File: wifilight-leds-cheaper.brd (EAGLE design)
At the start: 50.8 x 50.8 mm, 60 parts, among them Q3 FDN335N, Q4 FDN335N, Q5 FDN335N, Q6 FDN335N, U2 PCA9685

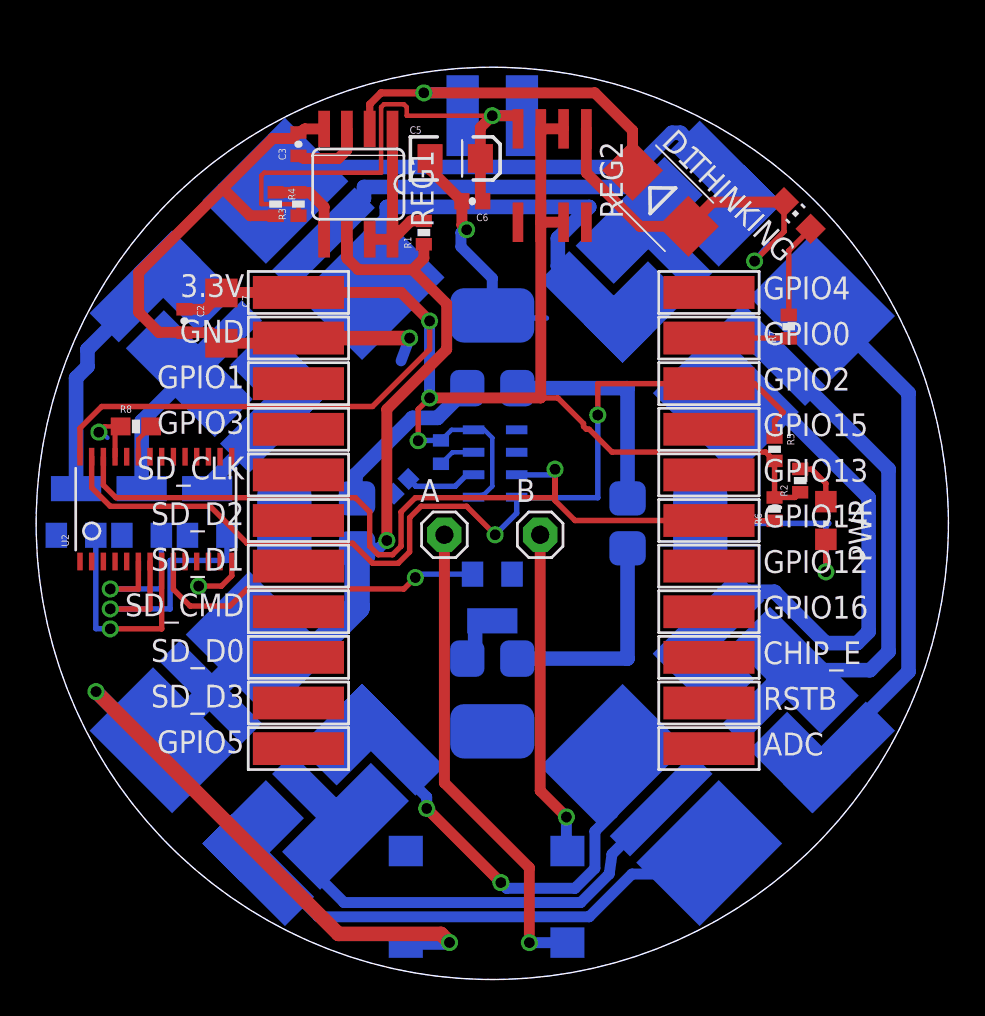
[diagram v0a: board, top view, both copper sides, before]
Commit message: Mk2
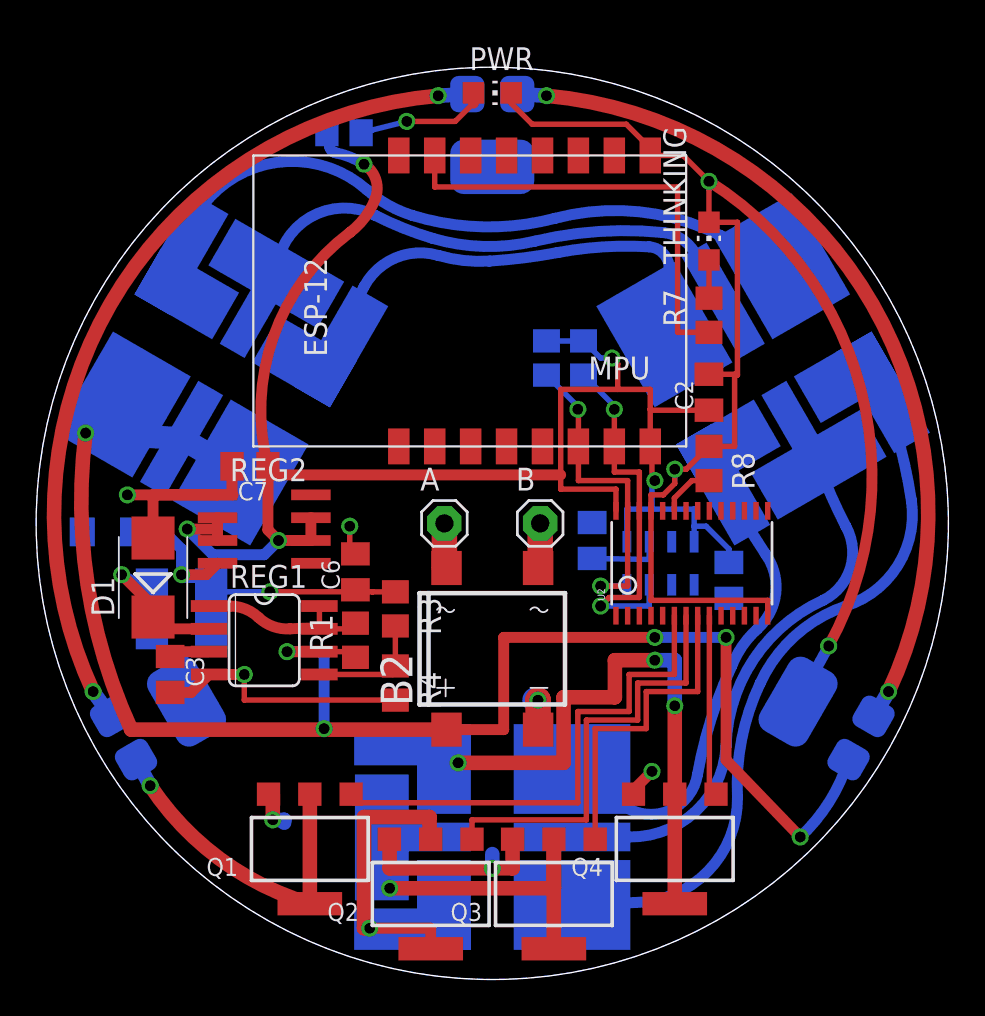
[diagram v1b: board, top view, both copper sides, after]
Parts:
- removed 3.3V, ADC, CHIP_E, GND, GPIO0, GPIO1, GPIO12, GPIO13, GPIO14, GPIO15, GPIO16, GPIO2, GPIO3, GPIO4, GPIO5, RSTB, SD_CLK, SD_CMD, SD_D0, SD_D1, SD_D2, SD_D3: WIREPADSMD5-1,8, wirepad:5-1,8
- removed LED4: OVSTRGBBCR8, led:OVSTRGBBCR8
- removed Q5, Q6: FDN335N, adafruit:SOT23-W
- removed U$4: LUXEON-REBEL, SparkFun-LED:LUXEON-REBEL
- added MPU: ESP8266_ESP-12, ESP8266-ESP12:ESP8266-ESP12
- added Q1, Q2: BUK98180-100A, nxp_60:SOT223
- C1, C2, C3: device SparkFun-Passives:0402-CAP -> resistor:C0805K
- C4, C6: device SparkFun-Capacitors:0402-CAP -> resistor:C0805K
- C7: device SparkFun-Capacitors:1206 -> resistor:C0805K
- Q3, Q4: value FDN335N -> BUK98180-100A; device adafruit:SOT23-W -> nxp_60:SOT223
- R1, R2, R3, R4, R5, R6, R7: device SparkFun-Passives:0402-RES -> resistor:R0805
- R8: device SparkFun-Resistors:0603-RES -> resistor:R0805
- moved D1 35.3 mm to (6.51, 22.4), turned to 90 degrees
- moved LED3 32.5 mm to (25.4, 7.94), turned to 0 degrees
- moved L1 32.5 mm to (8.10, 20.6)
- moved R8 32.0 mm to (37.5, 28.7), turned to 270 degrees
- moved R2 31.9 mm to (17.1, 47.1), flipped to the bottom, turned to 180 degrees
- moved Q3 31.3 mm to (28.8, 4.76), flipped to the top, turned to 180 degrees
- moved C3 30.4 mm to (7.46, 17.0), turned to 270 degrees
- moved U$3 30.3 mm to (7.14, 14.8), turned to 240 degrees
- moved U$1 30.3 mm to (43.7, 14.8), turned to 120 degrees
- moved PWR 30.2 mm to (25.4, 49.4), turned to 270 degrees
- moved U2 30.0 mm to (36.5, 23.2)
- moved C2 29.5 mm to (37.5, 32.7), turned to 90 degrees
- moved C5 28.4 mm to (3.97, 24.9), flipped to the bottom, turned to 180 degrees
- moved R4 27.5 mm to (20.0, 16.5)
- moved REG1 25.9 mm to (12.7, 18.9), turned to 270 degrees
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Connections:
- removed net N$12: U$3.CATHODE, U$4.ANODE
- removed net N$3: LED3.4, LED3.4@1, LED4.1
- removed net N$4: LED3.5, LED3.5@1, LED4.2
- removed net N$9: LED3.6, LED3.6@1, LED4.3
- new net N$25: MPU.13
- new net N$26: MPU.12
- new net N$27: MPU.11
- new net N$28: MPU.10
- new net N$29: MPU.9
- new net N$32: MPU.6
- new net N$33: MPU.4
- new net N$34: MPU.3
- new net N$35: MPU.2
- new net N$36: MPU.5
- net 3.3V: now also MPU.16; no longer 3.3V.1
- net BLUE: now also Q2.1; no longer Q5.1
- net GND: now also MPU.1, Q1.3, Q2.3, Q3.3, Q4.3; no longer GND.1, Q3.2, Q4.2, Q5.2, Q6.2, U$4.P$3
- net GREEN: now also Q4.1, U2.9; no longer Q6.1, U2.8
- net P_BLUE: now also LED3.6, LED3.6@1, Q2.2, Q2.4; no longer LED4.6, LED4.6@1, Q5.3
- net P_GREEN: now also LED3.4, LED3.4@1, Q4.2, Q4.4; no longer LED4.4, LED4.4@1, Q6.3
- net P_RED: now also LED3.5, LED3.5@1, Q3.2, Q3.4; no longer LED4.5, LED4.5@1, Q3.3
- net P_WHITE: now also Q1.2, Q1.4, U$3.CATHODE; no longer Q4.3, U$4.CATHODE
- net RED: now also U2.8; no longer U2.6
- net RESET: now also MPU.8; no longer GPIO4.1
- net SCL: now also MPU.15; no longer GPIO14.1
- net SDA: now also MPU.14; no longer GPIO2.1
- net THINKING: now also MPU.7; no longer GPIO0.1
- net WHITE: now also Q1.1, U2.6; no longer Q4.1, U2.9
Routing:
- net SDA: track 55.1 -> 18.3 mm
- net GND: track 92.9 -> 129.0 mm, vias 6 -> 10
- net 12V: track 77.6 -> 110.6 mm, vias 3 -> 6
- net N$10: track 9.60 -> 41.5 mm, vias 0 -> 2
- net SCL: track 50.4 -> 20.7 mm, vias 1 -> 2
- net N$11: track 12.3 -> 41.7 mm, vias 0 -> 2
- net N$3: track 28.7 -> 0.00 mm
- net N$18: track 26.8 -> 2.60 mm, vias 1 -> 0
- net N$9: track 23.2 -> 0.00 mm
- net N$4: track 22.0 -> 0.00 mm
- net P_GREEN: track 12.9 -> 34.1 mm, vias 0 -> 3
- net THINKING: track 4.45 -> 25.1 mm
- net N$19: track 18.3 -> 2.60 mm, vias 1 -> 0
- net P_WHITE: track 3.28 -> 18.8 mm, vias 0 -> 1
- net P_RED: track 7.50 -> 21.2 mm, vias 0 -> 1
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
